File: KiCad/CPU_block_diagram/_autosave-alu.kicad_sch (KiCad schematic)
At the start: 8 parts, among them U16 74LS245, U17 74LS283, U18 74LS283, U19 74LS86, U20 74LS86, U21 74LS02, U22 74LS08

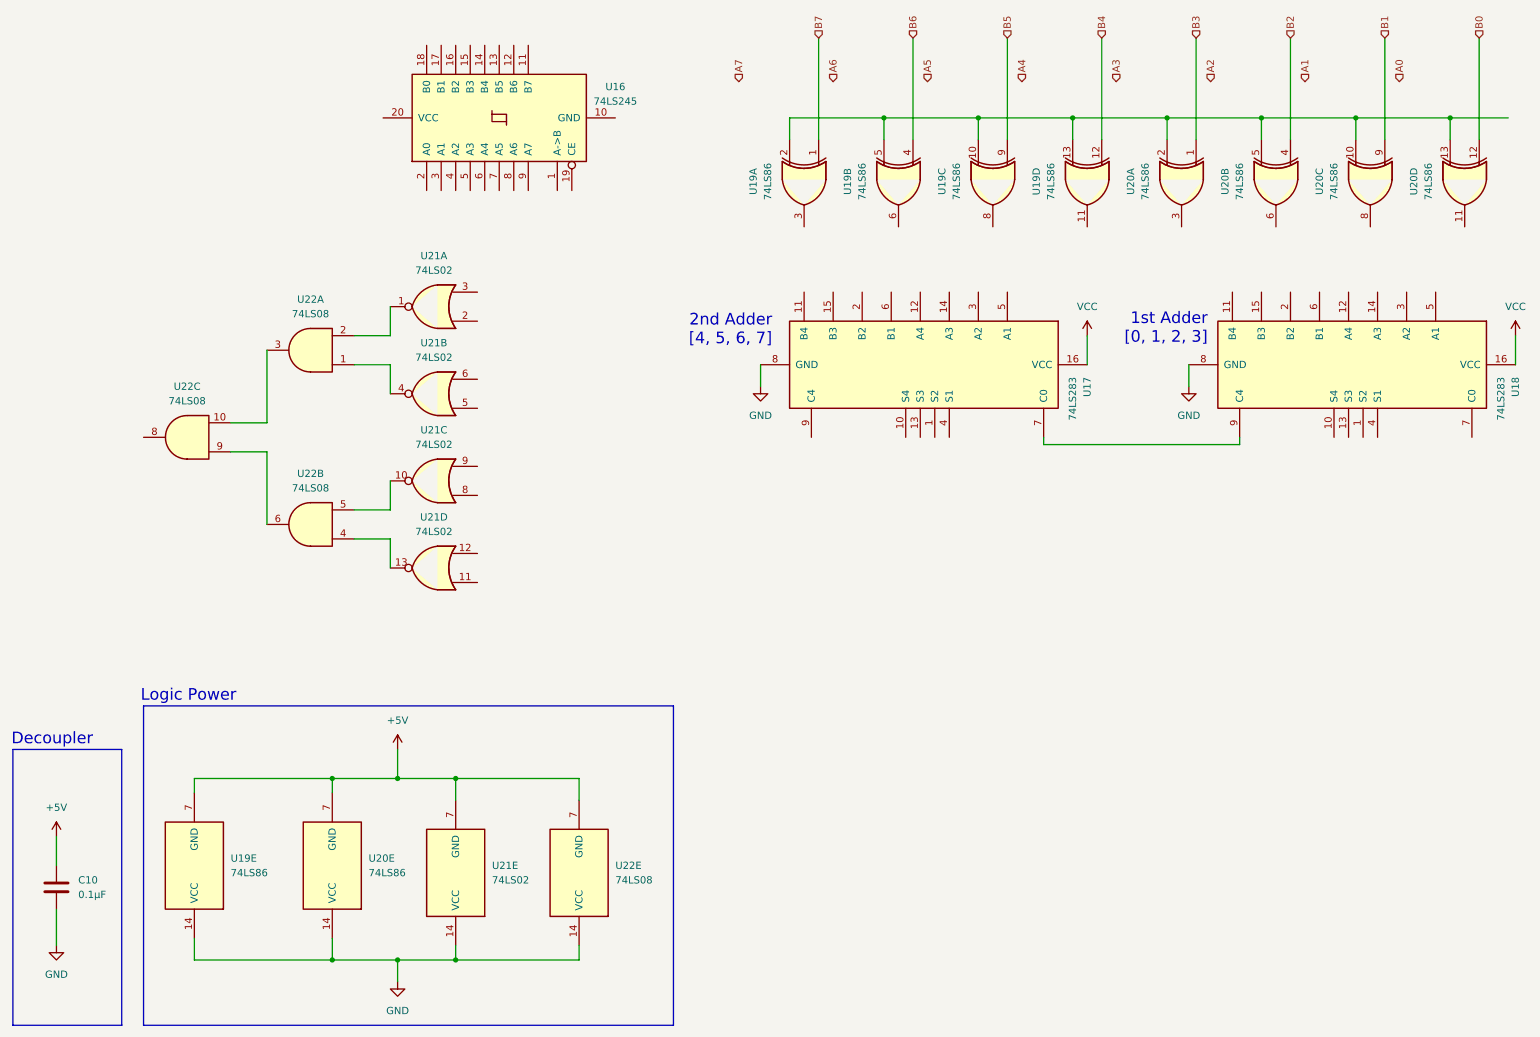
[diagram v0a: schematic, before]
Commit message: vault backup: 2026-01-15 13:45:16
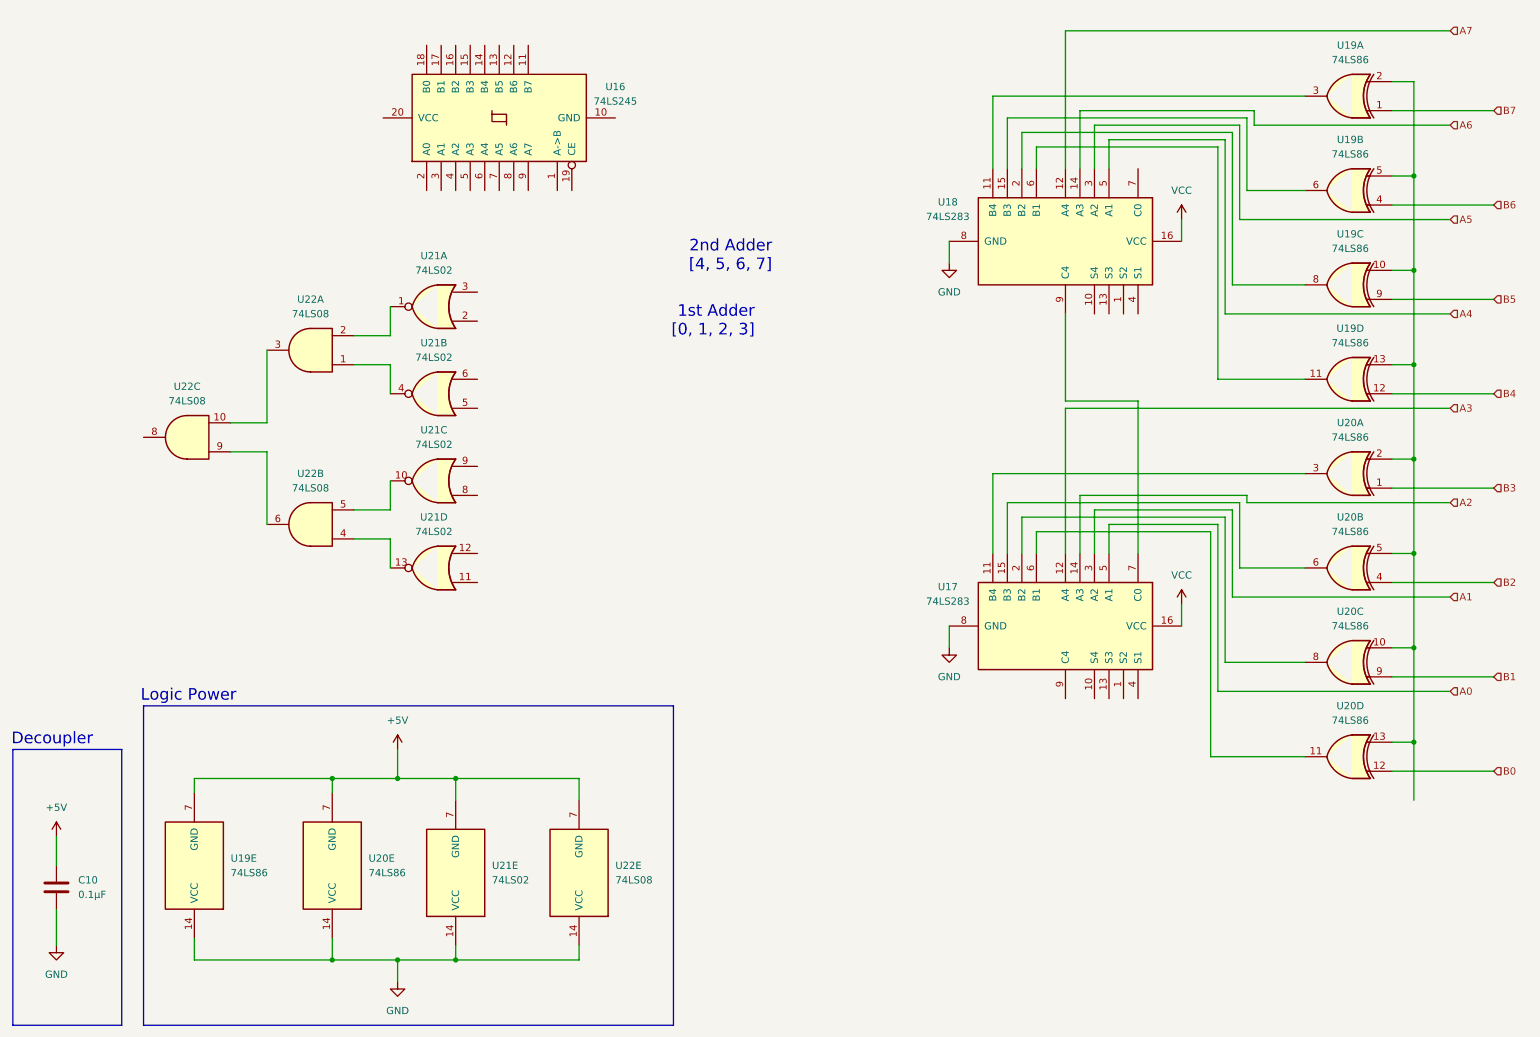
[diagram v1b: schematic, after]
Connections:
- net A0: now also U17.5 (A1)
- net A1: now also U17.3 (A2)
- net A2: now also U17.14 (A3)
- net A3: now also U17.12 (A4)
- net A4: now also U18.5 (A1)
- net A5: now also U18.3 (A2)
- net A6: now also U18.14 (A3)
- net A7: now also U18.12 (A4)
- net at U20.6: now also U17.15 (B3)
- net at U19.11: now also U18.6 (B1)
- net at U18.11 (B4): now also U19.3
- net at U18.15 (B3): now also U19.6
- net at U18.2 (B2): now also U19.8
- net at U17.11 (B4): now also U20.3
- net at U17.2 (B2): now also U20.8
- net at U17.6 (B1): now also U20.11
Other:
- moved on the sheet: U19A, U19B, U19C, U19D, U20A, U20B, U20C, U20D
